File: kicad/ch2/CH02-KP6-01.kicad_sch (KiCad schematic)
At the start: 7 parts

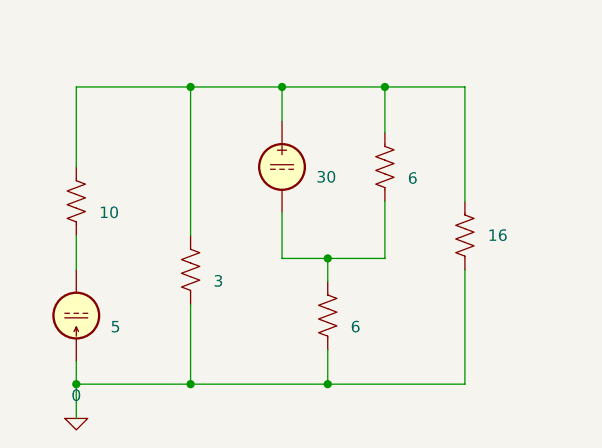
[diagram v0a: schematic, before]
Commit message: regular
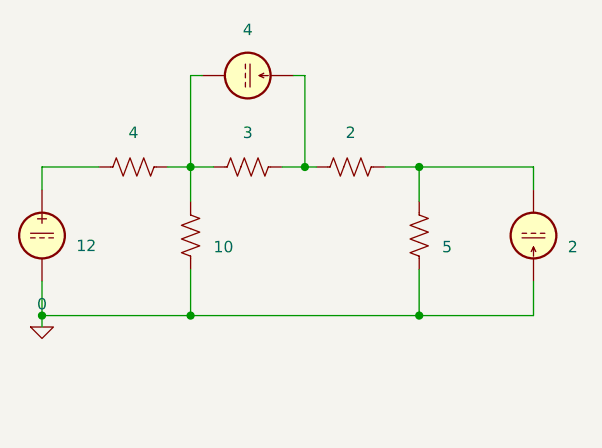
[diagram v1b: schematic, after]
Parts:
- removed I6: 5, symbol Simulation_SPICE:IDC
- removed R29: 10, symbol Device:R_US
- removed R30: 3, symbol Device:R_US
- removed R31, R32: 6, symbol Device:R_US
- removed R33: 16, symbol Device:R_US
- removed V12: 30, symbol Simulation_SPICE:VDC
- added I10: 4, symbol Simulation_SPICE:IDC
- added I9: 2, symbol Simulation_SPICE:IDC
- added R54: 4, symbol Device:R_US
- added R55: 3, symbol Device:R_US
- added R56: 2, symbol Device:R_US
- added R57: 10, symbol Device:R_US
- added R58: 5, symbol Device:R_US
- added V19: 12, symbol Simulation_SPICE:VDC
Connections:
- net 0: now also I9.1, R57.1, R58.1, V19.2
- new net: R54.1, V19.1
- new net: I10.2, R54.2, R55.1, R57.2
- new net: I10.1, R55.2, R56.1
- new net: I9.2, R56.2, R58.2
